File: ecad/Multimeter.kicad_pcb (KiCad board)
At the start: 2 copper layers, 68 x 110 mm, 88 parts, among them J1 USB_B_Micro, J3 Red Banana Plug, J4 Black Banana Plug, Q1 2N7002, Q10 BSS84, Q11 BSS84, Q12 2N7002, Q13 BSS84, Q14 2N7002, Q15 2N7002, Q16 2N7002, Q2 2N7002, Q3 2N7002, Q4 2N7002, Q5 BSS84, Q6 BSS84, Q7 BSS84, Q8 BSS84, Q9 BSS84, SW3 GF-126-0159, SW4 GF-123-0054, U1 SC0915, U10 MCP3561, U2 4021, U3 OPA4388IDR, U6 812, U7 LM4030-2.5

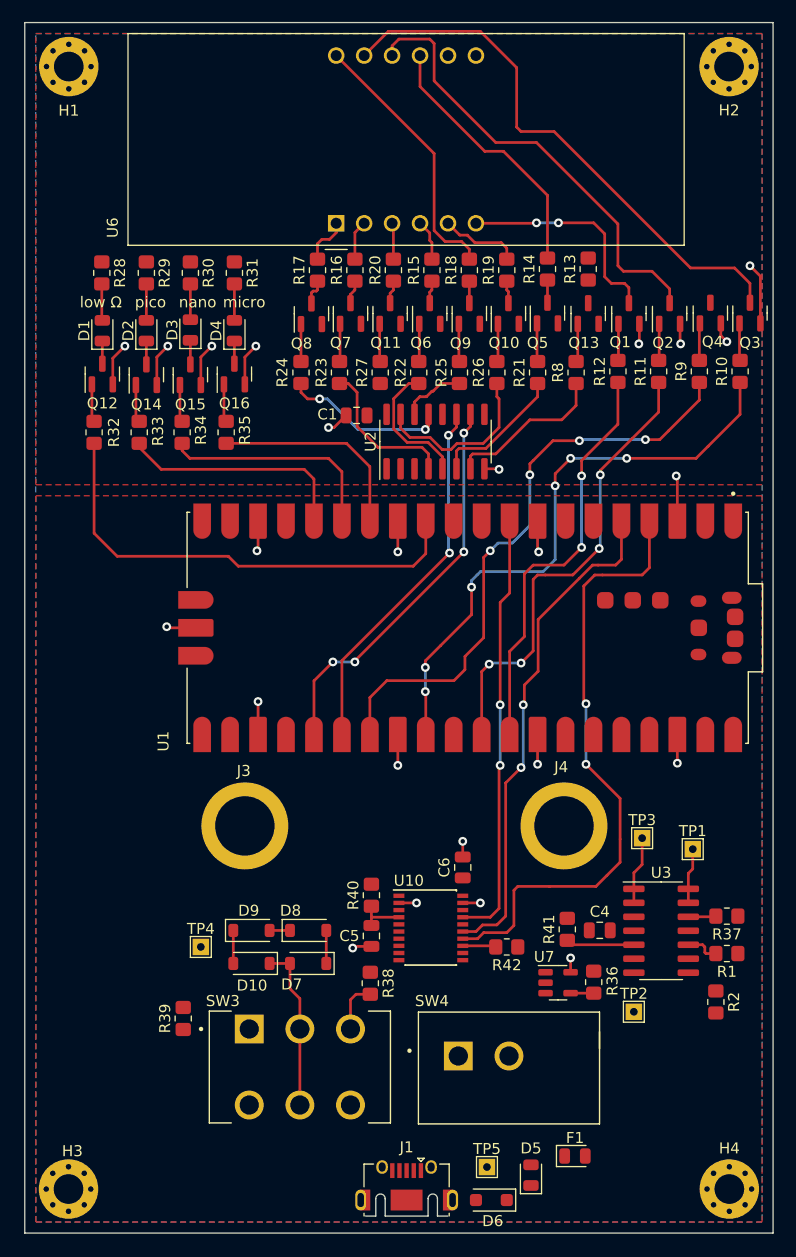
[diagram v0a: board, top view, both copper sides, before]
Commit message: layout finished
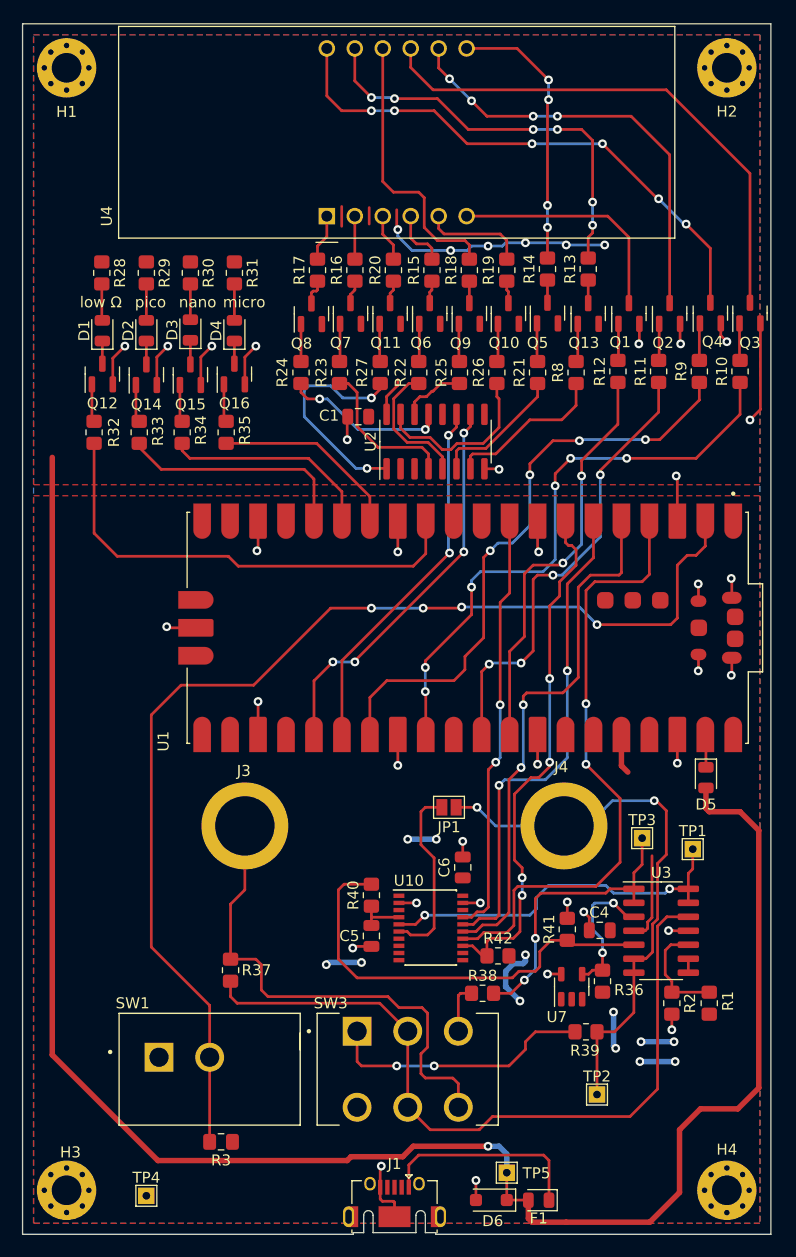
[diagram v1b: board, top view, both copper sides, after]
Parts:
- removed D10, D7, D8, D9: 1N4148W, Diode_SMD:D_SOD-123
- removed SW4: GF-123-0054, Multimeter:SW_GF-123-0054
- removed U6: 812, Display_7Segment:CA56-12EWA
- added JP1: ~, Jumper:SolderJumper-2_P1.3mm_Open_Pad1.0x1.5mm, F.Cu at (146.8, 106.2)
- added R3: 10k, Capacitor_SMD:C_0805_2012Metric_Pad1.18x1.45mm_HandSolder, F.Cu at (126.0, 136.6)
- added SW1: GF-123-0054, Multimeter:SW_GF-123-0054, F.Cu at (125.0, 130.0)
- added U4: CC56-12SURKWA, Display_7Segment:CA56-12SURKWA, F.Cu at (135.7, 52.5)
- D1, D2, D3, D4: value LTST-C171TBKT -> LTST-C170KRKT
- R13, R14, R15, R16, R17, R18, R19, R20: value 442 -> 649
- R28, R29, R30, R31: value 383 -> 649
- R37: value 1.43M+/-0.1% -> 500k+/-0.1%
- moved R37 45.4 mm to (126.9, 121.0), turned to -90 degrees
- moved D5 39.5 mm to (170.1, 103.5), turned to -90 degrees
- moved R39 36.6 mm to (159.2, 126.6), turned to 0 degrees
- moved TP4 23.1 mm to (119.2, 141.5)
- moved R38 10.2 mm to (149.8, 123.1), turned to 180 degrees
- moved SW3 9.80 mm to (143.0, 130.0)
- moved TP2 8.23 mm to (160.2, 132.3)
- moved F1 5.20 mm to (154.9, 141.9), turned to 180 degrees
- moved R1 4.79 mm to (170.4, 124.0), turned to 90 degrees
- moved R2 4.00 mm to (167.0, 124.0)
- moved TP5 1.87 mm to (152.0, 139.4)
- moved J1 1.87 mm to (141.8, 143.4)
- moved U7 1.29 mm to (157.9, 122.5), turned to 90 degrees
- moved R42 1.14 mm to (151.2, 119.7)
- moved R36 0.80 mm to (160.7, 122.0), turned to 90 degrees
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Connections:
- J4 pad 1: Net-(D8-K) -> Net-(J4-Pin_1)
- R39 pad 2: Net-(SW4-B) -> Net-(J4-Pin_1)
- TP2 pad 1: Net-(D8-K) -> Net-(J4-Pin_1)
- U1 pad 2: unconnected-(U1-GP1-Pad2) -> Net-(SW1-B)
- U1 pad 36: unconnected-(U1-3V3_OUT-Pad36) -> +3.3V
- U10 pad 6: unconnected-(U10-CH1-Pad6) -> Net-(JP1-B)
- U3 pad 6: Net-(D8-K) -> Net-(J4-Pin_1)
- U3 pad 7: Net-(D8-K) -> Net-(J4-Pin_1)
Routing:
- net +5V: track 0.00 -> 197.6 mm, vias 0 -> 7
- net Net-(SW1-B): track 0.00 -> 104.1 mm, vias 0 -> 4
- net Net-(U3D-+): track 17.6 -> 68.7 mm
- net Net-(J4-Pin_1): track 0.00 -> 51.1 mm, vias 0 -> 2
- net Net-(Q4-D): track 0.00 -> 49.8 mm, vias 0 -> 6
- net Net-(J3-Pin_1): track 0.00 -> 45.6 mm
- net /Analog Front End/CS: track 3.04 -> 48.2 mm, vias 0 -> 4
- net /Analog Front End/SDO: track 0.00 -> 45.2 mm, vias 0 -> 2
- net Net-(U4-a): track 0.00 -> 37.7 mm, vias 0 -> 6
- net +3.3V: track 0.00 -> 33.3 mm, vias 0 -> 12
- net Net-(U3B-+): track 6.22 -> 39.5 mm
- net Net-(U10-CH0): track 5.04 -> 33.8 mm, vias 0 -> 2
- net Net-(R39-Pad1): track 0.00 -> 24.4 mm, vias 0 -> 2
- net GND: track 64.3 -> 88.7 mm, vias 24 -> 34
- net Net-(U3A--): track 6.19 -> 26.6 mm, vias 0 -> 2
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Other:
- outline, holes or cut-outs redrawn
